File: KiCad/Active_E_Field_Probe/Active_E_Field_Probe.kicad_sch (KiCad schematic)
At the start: 13 parts

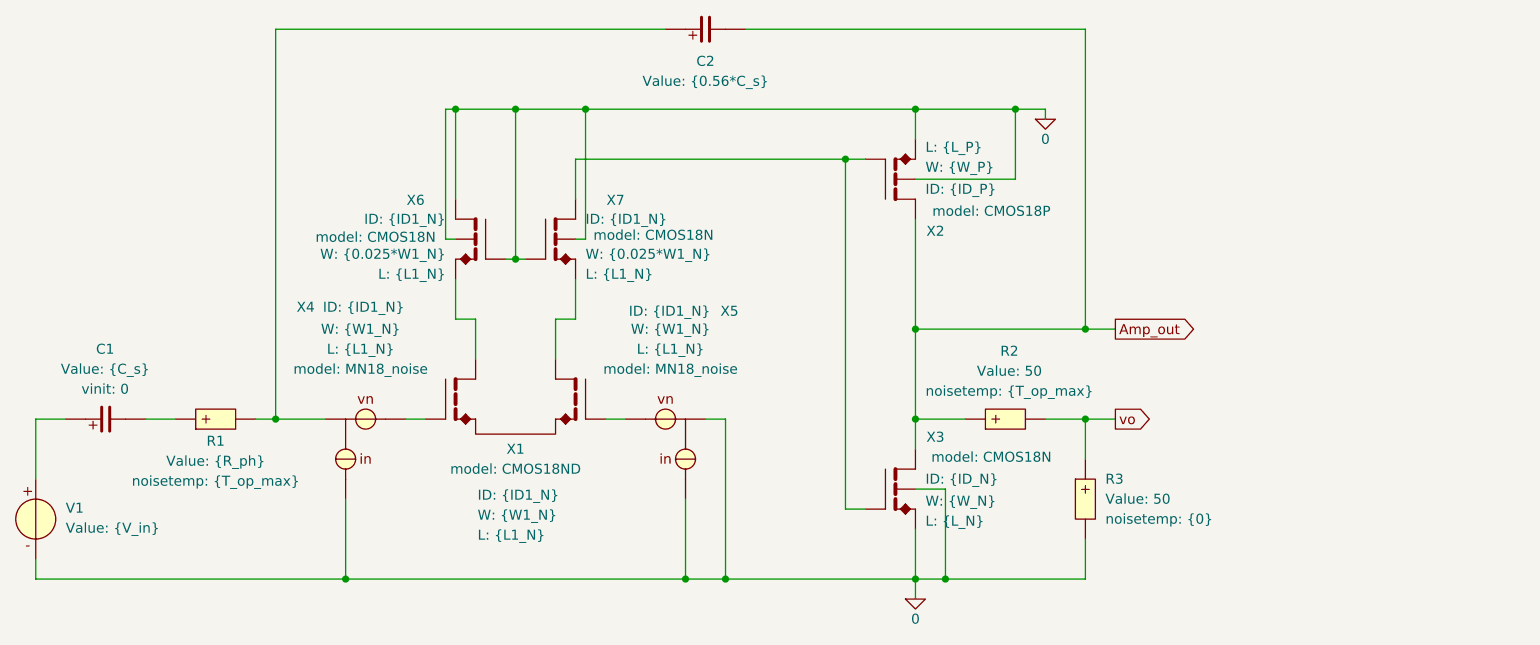
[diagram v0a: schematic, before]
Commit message: push
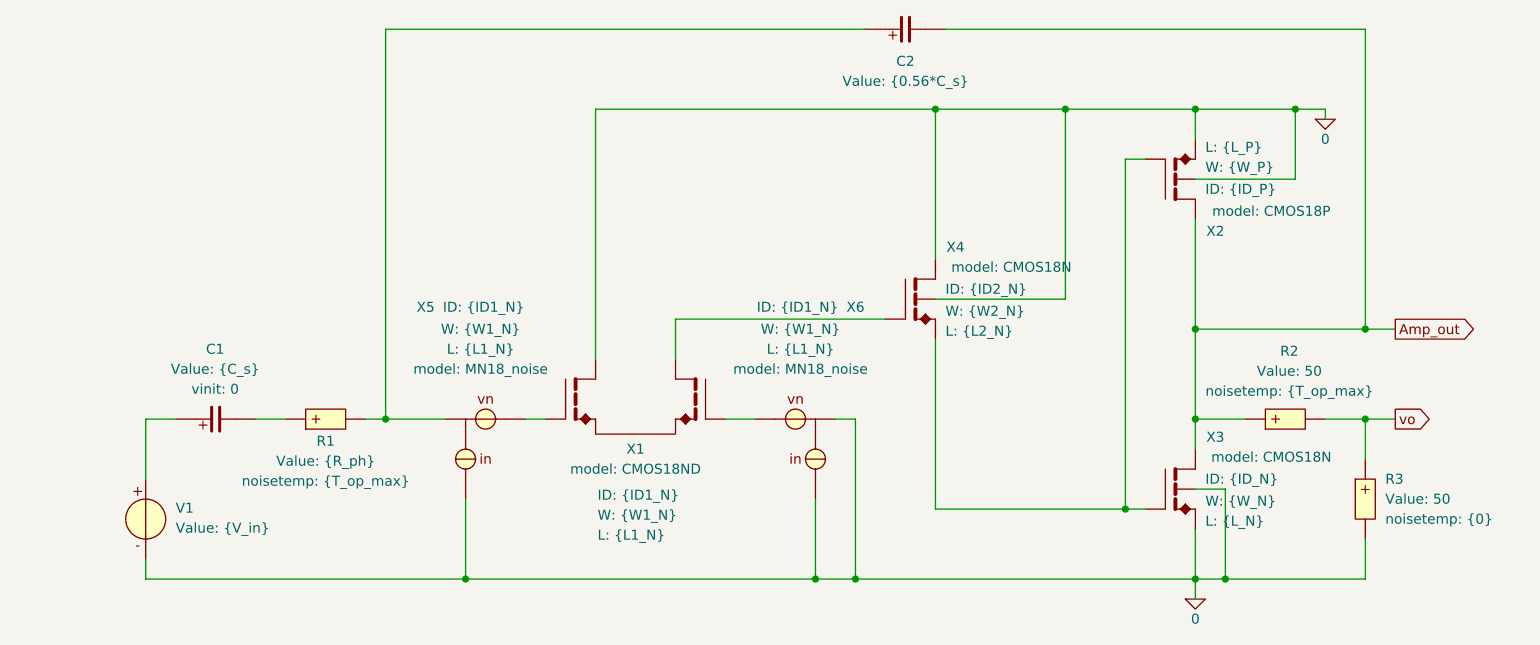
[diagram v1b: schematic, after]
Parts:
- removed X5: ~, symbol SLiCAP:M_noise
- removed X6, X7: ~, symbol SLiCAP:XM
- added X4: ~, symbol SLiCAP:XM
- added X6: ~, symbol SLiCAP:M_noise
- renumbered X4 to X5
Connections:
- net 0: now also X1.1 (D1), X4.1 (D), X4.4 (B), X6.1 (ext), X6.2 (comm)
- net at X2.2 (G), X3.2 (G): now also X4.3 (S)
- net at X1.2 (D2): now also X4.2 (G)
- net at X1.4 (G2): now also X6.3 (int)
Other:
- moved on the sheet: C1, C2, R1, R2, R3, V1, X1, X2, X3, X5
